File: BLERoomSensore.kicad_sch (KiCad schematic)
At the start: 16 parts, among them J2 Conn_ARM_SWD_TagConnect_TC203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, U2 BME280, U3 BMD-360-A-R, U4 LIS2DH12TR, U5 PCF8523T

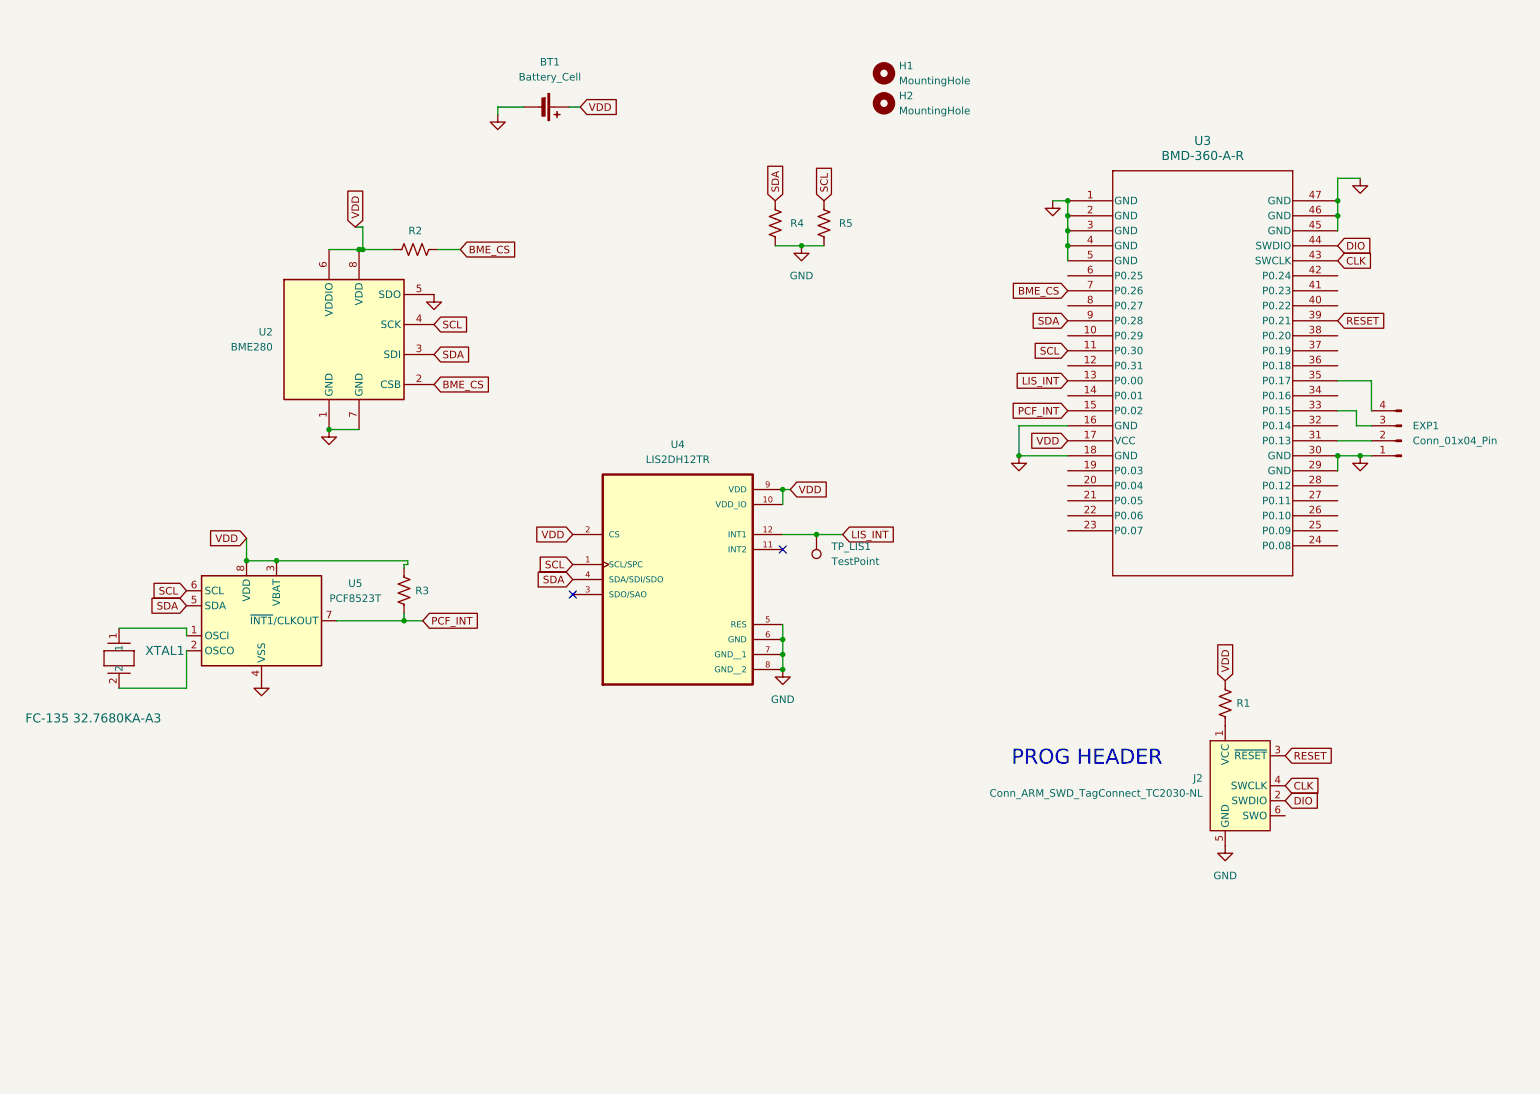
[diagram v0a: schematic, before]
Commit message: Working on comp changes
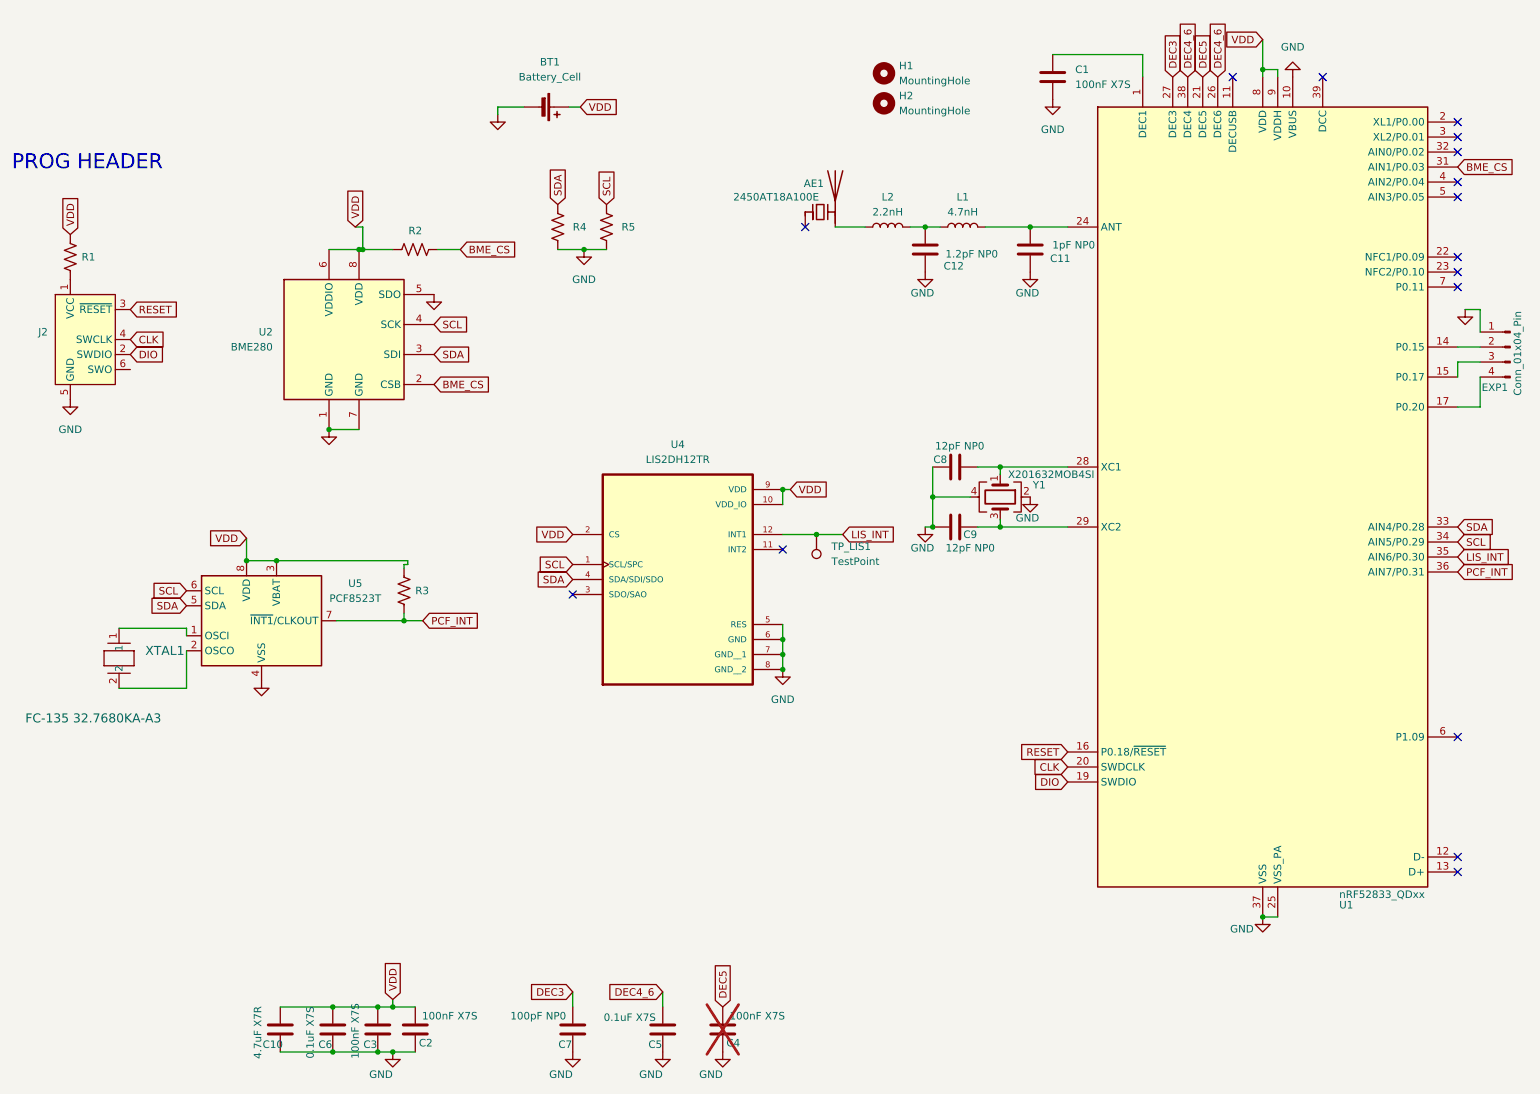
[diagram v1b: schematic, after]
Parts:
- removed U3: BMD-360-A-R, BMD-360_UBL, symbol BMD-360-A-R:BMD-360-A-R
- added AE1: 2450AT18A100E, Capacitor_SMD:C_0603_1608Metric, symbol Device:Antenna_Chip
- added C1, C2, C3, C4: 100nF X7S, Capacitor_SMD:C_0402_1005Metric_Pad0.74x0.62mm_HandSolder, symbol Device:C
- added C10: 4.7uF X7R, Capacitor_SMD:C_0603_1608Metric_Pad1.08x0.95mm_HandSolder, symbol Device:C
- added C11: 1pF NP0, Capacitor_SMD:C_0402_1005Metric_Pad0.74x0.62mm_HandSolder, symbol Device:C
- added C12: 1.2pF NP0, Capacitor_SMD:C_0402_1005Metric_Pad0.74x0.62mm_HandSolder, symbol Device:C
- added C5, C6: 0.1uF X7S, Capacitor_SMD:C_0402_1005Metric_Pad0.74x0.62mm_HandSolder, symbol Device:C
- added C7: 100pF NP0, Capacitor_SMD:C_0402_1005Metric_Pad0.74x0.62mm_HandSolder, symbol Device:C
- added C8, C9: 12pF NP0, Capacitor_SMD:C_0402_1005Metric_Pad0.74x0.62mm_HandSolder, symbol Device:C
- added L1: 4.7nH, Inductor_SMD:L_0402_1005Metric, symbol Device:L
- added L2: 2.2nH, Inductor_SMD:L_0402_1005Metric, symbol Device:L
- added U1: nRF52833_QDxx, Package_DFN_QFN:QFN-40-1EP_5x5mm_P0.4mm_EP3.6x3.6mm, symbol MCU_Nordic:nRF52833_QDxx
- added Y1: X201632MOB4SI, Crystal:Crystal_SMD_2016-4Pin_2.0x1.6mm, symbol Device:Crystal_GND24
- EXP1: footprint Connector_PinHeader_1.00mm:PinHeader_1x04_P1.00mm_Vertical -> Connector_PinHeader_1.27mm:PinHeader_1x04_P1.27mm_Vertical
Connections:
- net BME_CS: now also U1.31 (AIN1/P0.03)
- net CLK: now also U1.20 (SWDCLK)
- net DIO: now also U1.19 (SWDIO)
- net GND: now also C1.2, C10.1, C11.1, C12.1, C2.1, C3.1, C4.1, C5.1, C6.1, C7.1, C8.1, C9.2, U1.10 (VBUS), U1.25 (VSS_PA), U1.37 (VSS), U1.41 (VSS), Y1.2, Y1.4
- net LIS_INT: now also U1.35 (AIN6/P0.30)
- net PCF_INT: now also U1.36 (AIN7/P0.31)
- net RESET: now also U1.16 (P0.18/~{RESET})
- net SCL: now also U1.34 (AIN5/P0.29)
- net SDA: now also U1.33 (AIN4/P0.28)
- net VDD: now also C10.2, C2.2, C3.2, C6.2, U1.18 (VDD), U1.30 (VDD), U1.40 (VDD), U1.8 (VDD), U1.9 (VDDH)
- net at EXP1.2 (Pin_2): now also U1.14 (P0.15)
- net at EXP1.3 (Pin_3): now also U1.15 (P0.17)
- net at EXP1.4 (Pin_4): now also U1.17 (P0.20)
- new net: C1.1, U1.1 (DEC1)
- new net: C11.2, L1.2, U1.24 (ANT)
- new net: C8.2, U1.28 (XC1), Y1.1
- new net: C9.1, U1.29 (XC2), Y1.3
- new net: AE1.2 (PCB_Trace), L2.1
- new net: C12.2, L1.1, L2.2
- new net DEC3: C7.2, U1.27 (DEC3)
- new net DEC4_6: C5.2, U1.26 (DEC6), U1.38 (DEC4)
- new net DEC5: C4.2, U1.21 (DEC5)
- no-connect marks 2 -> 16
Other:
- moved on the sheet: J2, R1, R4, R5
